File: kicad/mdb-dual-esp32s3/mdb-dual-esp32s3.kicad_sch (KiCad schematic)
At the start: 52 parts, among them J1 MDB_Connector, J2 USB_C_Receptacle_USB2.0_16P, J4 Conn_Coaxial, J8 Conn_01x04_Pin, J9 MDB_Connector, Q8 MMBT3904, SW1 SW_Push, U1 TLP785, U3 ESP32-S3FH4R2, U4 TLP785, U5 LM2594HVM-3.3, U7 MT3608, Y1 Crystal_GND24

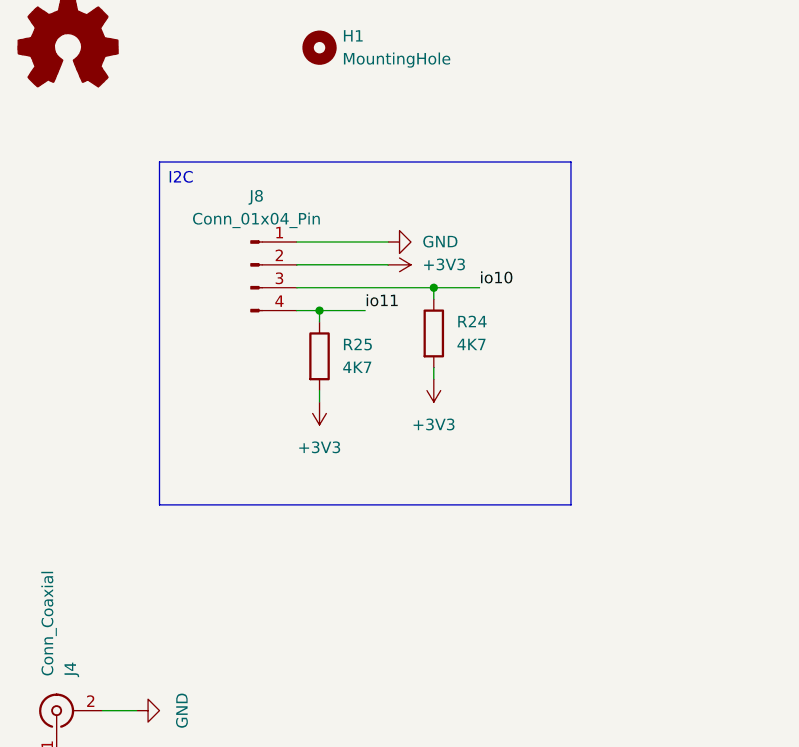
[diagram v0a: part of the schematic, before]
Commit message: routing
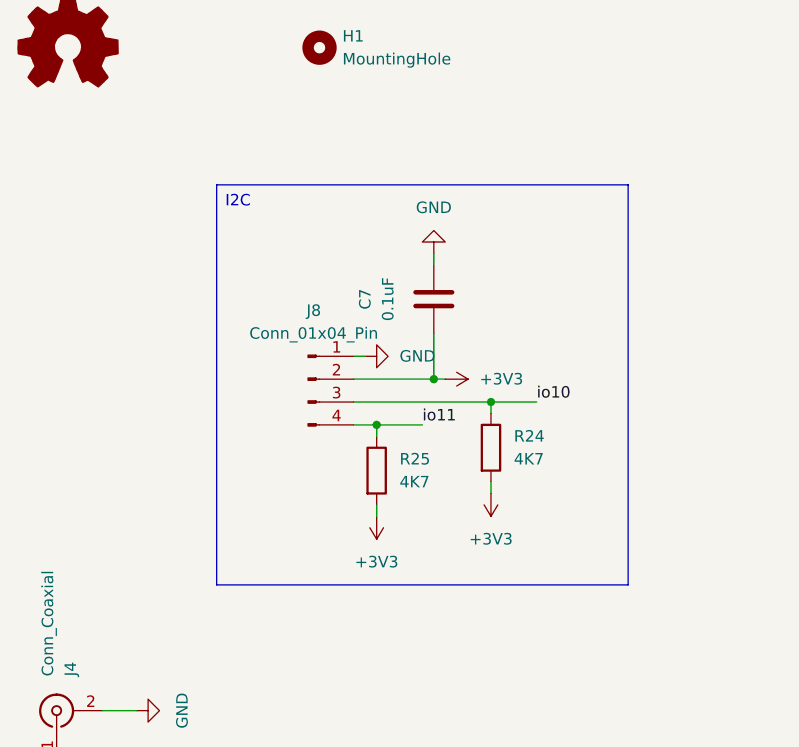
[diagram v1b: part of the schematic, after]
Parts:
- added C7: 0.1uF, Capacitor_SMD:C_0603_1608Metric, symbol Device:C
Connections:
- net +3V3: now also C7.1
- net GND: now also C7.2
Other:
- moved on the sheet: J8, R24, R25
